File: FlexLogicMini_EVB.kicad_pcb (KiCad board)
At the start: 8 copper layers, 50 x 50 mm, 183 parts, among them IC1 SL2.1s, IC2 MT9700, IC3 MTS4P, IC4 LCMXO2-1200HC-4SG32I, IC5 W25Q16JVUXIQ, J1 GT-USB-7010ASV, J10 Conn_02x03_Odd_Even, J11 Conn_01x04, J12 1.0-3PWB, J13 1.0-3PWB, J2 WJ126V-5.0-2P, J3 WJ126V-5.0-2P, J4 WJ126V-5.0-2P, J5 WJ126V-5.0-2P, J6 Conn_02x03_Odd_Even, J7 Conn_02x03_Odd_Even, J8 Conn_02x03_Odd_Even, J9 Conn_02x03_Odd_Even, SW1 DSWB02LHGETB, U1 ADS1115IDGSR, U10 RP2040, U11 TMUX1574DYYR, U2 ADS1115IDGSR, U3 RQ12000160, U4 RT5752BHGJ5, U5 93LC56BT-I, U6 RQ12000160, U7 FT2232HL, U8 RQ12000160, U9 TLV803SDBZR

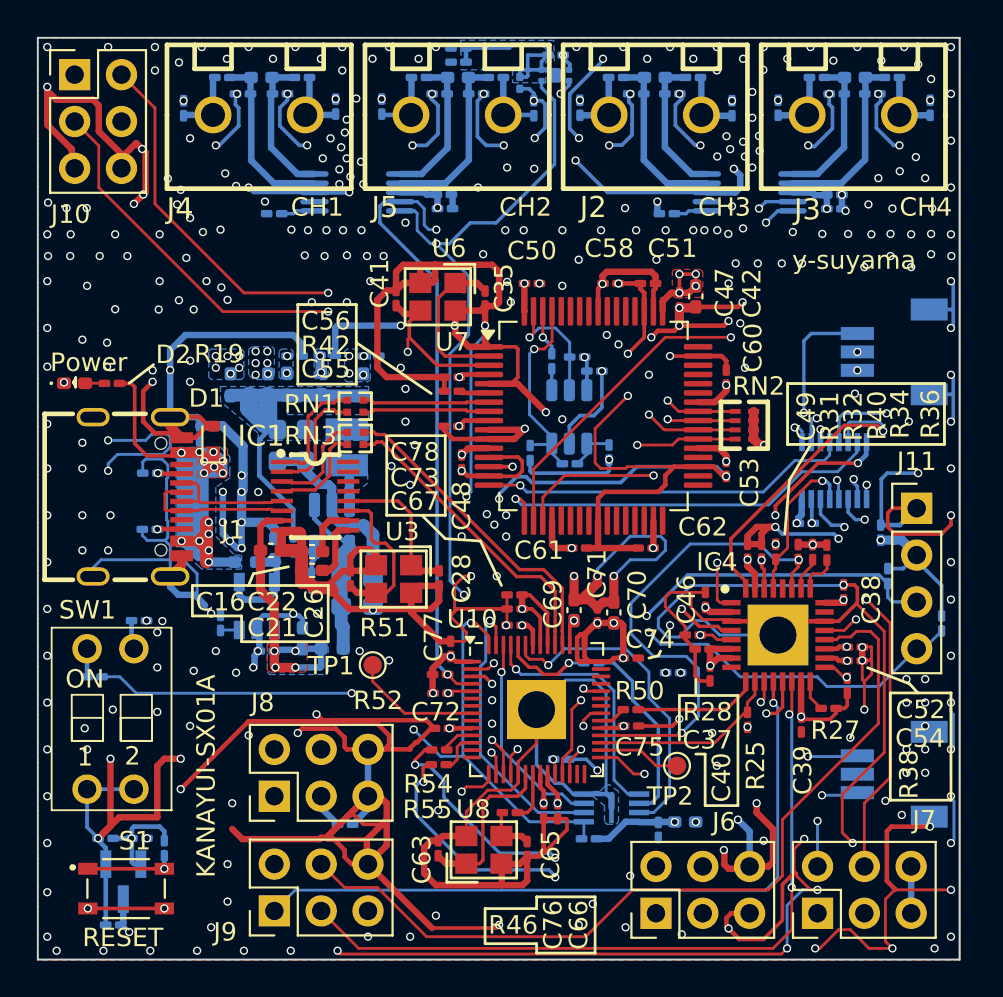
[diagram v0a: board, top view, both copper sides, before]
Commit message: V3 commit
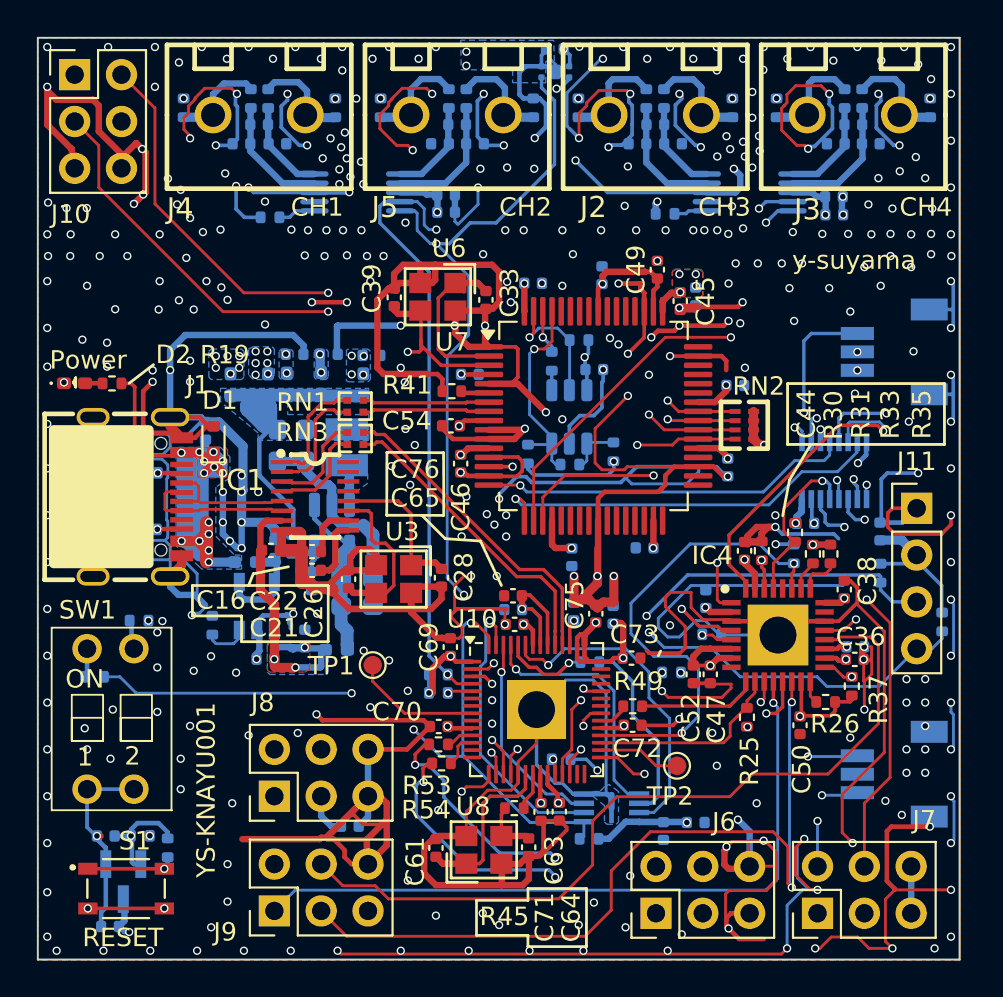
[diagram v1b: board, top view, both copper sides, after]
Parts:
- removed the C31 at (134.3, 72.3)
- removed the C34 at (141.7, 89.1)
- removed the C40 at (148.0, 105.5)
- removed the C66 at (139.7, 113.0)
- removed C78, C79: 0.1uF, Capacitor_SMD:C_0201_0603Metric_Pad0.64x0.40mm_HandSolder
- removed the R27 at (154.4, 107.4)
- removed the R36 at (154.3, 98.9)
- removed the R40 at (152.7, 98.9)
- removed the R52 at (133.3, 106.6)
- removed the R55 at (133.3, 110.4)
- added C33: 33pF, Capacitor_SMD:C_0402_1005Metric, F.Cu at (135.8, 85.2)
- added C36: 0.1uF, Capacitor_SMD:C_0402_1005Metric, F.Cu at (155.8, 104.7)
- added C42: 0.1uF, Capacitor_SMD:C_0402_1005Metric, B.Cu at (127.3, 88.2)
- added C68: 1uF, Capacitor_SMD:C_0402_1005Metric, B.Cu at (142.7, 102.3)
- added R30: 2.2k, Resistor_SMD:R_0402_1005Metric, F.Cu at (150.8, 98.8)
- added R37: 10k, Resistor_SMD:R_0402_1005Metric, F.Cu at (155.7, 106.2)
- added R44: 100, Resistor_SMD:R_0402_1005Metric, B.Cu at (145.9, 105.4)
- added R53: 100, Resistor_SMD:R_0402_1005Metric, F.Cu at (133.2, 109.3)
- C1, C10, C11, C12, C13, C14, C17, C18, C19, C20, C23, C25, C30, C38, C43, C46, C47, C49, C50, C52, C54, C59, C6, C7, C71, C72, C73, C75, C76, C8, C9: footprint Capacitor_SMD:C_0201_0603Metric_Pad0.64x0.40mm_HandSolder -> Capacitor_SMD:C_0402_1005Metric
- C15, C16, C2, C21, C22, C24, C3, C4, C5: footprint Capacitor_SMD:C_0402_1005Metric_Pad0.74x0.62mm_HandSolder -> Capacitor_SMD:C_0402_1005Metric
- C26, C28, C63: value 30pF -> 33pF; footprint Capacitor_SMD:C_0201_0603Metric_Pad0.64x0.40mm_HandSolder -> Capacitor_SMD:C_0402_1005Metric
- C32: value 1000pF -> 0.1uF; footprint Capacitor_SMD:C_0201_0603Metric -> Capacitor_SMD:C_0402_1005Metric
- C35, C41: value 30pF -> 0.1uF; footprint Capacitor_SMD:C_0201_0603Metric_Pad0.64x0.40mm_HandSolder -> Capacitor_SMD:C_0402_1005Metric; moved to B.Cu
- C37, C48, C51, C53, C56, C58, C60, C62, C74, C77: footprint Capacitor_SMD:C_0201_0603Metric_Pad0.64x0.40mm_HandSolder -> Capacitor_SMD:C_0402_1005Metric; moved to B.Cu
- C39, C61: value 0.1uF -> 33pF; footprint Capacitor_SMD:C_0201_0603Metric_Pad0.64x0.40mm_HandSolder -> Capacitor_SMD:C_0402_1005Metric
- C40: renamed from C42; footprint Capacitor_SMD:C_0402_1005Metric_Pad0.74x0.62mm_HandSolder -> Capacitor_SMD:C_0402_1005Metric; moved to B.Cu
- C44, C45, C64: footprint Capacitor_SMD:C_0201_0603Metric_Pad0.64x0.40mm_HandSolder -> Capacitor_SMD:C_0402_1005Metric; moved to F.Cu
- C55, C67: value 0.1uF -> 1uF; footprint Capacitor_SMD:C_0201_0603Metric_Pad0.64x0.40mm_HandSolder -> Capacitor_SMD:C_0402_1005Metric; moved to B.Cu
- C57, C69, C70: value 1uF -> 0.1uF; footprint Capacitor_SMD:C_0402_1005Metric_Pad0.74x0.62mm_HandSolder -> Capacitor_SMD:C_0402_1005Metric
- C65: value 30pF -> 0.1uF; footprint Capacitor_SMD:C_0201_0603Metric_Pad0.64x0.40mm_HandSolder -> Capacitor_SMD:C_0402_1005Metric
- C66: renamed from C68; footprint Capacitor_SMD:C_0201_0603Metric_Pad0.64x0.40mm_HandSolder -> Capacitor_SMD:C_0402_1005Metric
- R1, R17, R18, R19, R2, R20, R21, R22, R23, R24, R25, R3, R31, R39, R4, R5, R54, R6, R7, R8: footprint Resistor_SMD:R_0201_0603Metric_Pad0.64x0.40mm_HandSolder -> Resistor_SMD:R_0402_1005Metric
- R10, R11, R12, R13, R14, R15, R16, R9: value 240 -> 220; footprint Resistor_SMD:R_0201_0603Metric_Pad0.64x0.40mm_HandSolder -> Resistor_SMD:R_0402_1005Metric
- R26: value 0 -> 10k; footprint Resistor_SMD:R_0201_0603Metric_Pad0.64x0.40mm_HandSolder -> Resistor_SMD:R_0402_1005Metric; moved to F.Cu
- R27: renamed from R28; footprint Resistor_SMD:R_0201_0603Metric_Pad0.64x0.40mm_HandSolder -> Resistor_SMD:R_0402_1005Metric; moved to B.Cu
- R28: renamed from R29; footprint Resistor_SMD:R_0201_0603Metric_Pad0.64x0.40mm_HandSolder -> Resistor_SMD:R_0402_1005Metric
- R29: renamed from R30; footprint Resistor_SMD:R_0201_0603Metric_Pad0.64x0.40mm_HandSolder -> Resistor_SMD:R_0402_1005Metric
- R32: value 2.2k -> 10k; footprint Resistor_SMD:R_0201_0603Metric_Pad0.64x0.40mm_HandSolder -> Resistor_SMD:R_0402_1005Metric; moved to B.Cu
- R33, R35: value 10k -> 4.7k; footprint Resistor_SMD:R_0201_0603Metric_Pad0.64x0.40mm_HandSolder -> Resistor_SMD:R_0402_1005Metric; moved to F.Cu
- R34: value 4.7k -> 10k; footprint Resistor_SMD:R_0201_0603Metric_Pad0.64x0.40mm_HandSolder -> Resistor_SMD:R_0402_1005Metric; moved to B.Cu
- R36: renamed from R37; footprint Resistor_SMD:R_0201_0603Metric_Pad0.64x0.40mm_HandSolder -> Resistor_SMD:R_0402_1005Metric
- R38, R51: footprint Resistor_SMD:R_0201_0603Metric_Pad0.64x0.40mm_HandSolder -> Resistor_SMD:R_0402_1005Metric; moved to B.Cu
- R40: renamed from R41; value 30 -> 33; footprint Resistor_SMD:R_0201_0603Metric_Pad0.64x0.40mm_HandSolder -> Resistor_SMD:R_0402_1005Metric
- R41: renamed from R42; footprint Resistor_SMD:R_0201_0603Metric_Pad0.64x0.40mm_HandSolder -> Resistor_SMD:R_0402_1005Metric
- R42: renamed from R43; footprint Resistor_SMD:R_0201_0603Metric_Pad0.64x0.40mm_HandSolder -> Resistor_SMD:R_0402_1005Metric
- R43: renamed from R44; footprint Resistor_SMD:R_0201_0603Metric_Pad0.64x0.40mm_HandSolder -> Resistor_SMD:R_0402_1005Metric
- R45: value 100 -> 33; footprint Resistor_SMD:R_0201_0603Metric_Pad0.64x0.40mm_HandSolder -> Resistor_SMD:R_0402_1005Metric; moved to F.Cu
- R46: value 30 -> 33; footprint Resistor_SMD:R_0201_0603Metric_Pad0.64x0.40mm_HandSolder -> Resistor_SMD:R_0402_1005Metric; moved to B.Cu
- R47: value 30 -> 10k; footprint Resistor_SMD:R_0201_0603Metric_Pad0.64x0.40mm_HandSolder -> Resistor_SMD:R_0402_1005Metric
- R48: value 10k -> 33; footprint Resistor_SMD:R_0201_0603Metric_Pad0.64x0.40mm_HandSolder -> Resistor_SMD:R_0402_1005Metric
- R49: value 30 -> 33; footprint Resistor_SMD:R_0201_0603Metric_Pad0.64x0.40mm_HandSolder -> Resistor_SMD:R_0402_1005Metric; moved to F.Cu
- R50: value 30 -> 2.2k; footprint Resistor_SMD:R_0201_0603Metric_Pad0.64x0.40mm_HandSolder -> Resistor_SMD:R_0402_1005Metric; moved to B.Cu
- R52: renamed from R53; footprint Resistor_SMD:R_0201_0603Metric_Pad0.64x0.40mm_HandSolder -> Resistor_SMD:R_0402_1005Metric
- R55: renamed from R56; footprint Resistor_SMD:R_0201_0603Metric_Pad0.64x0.40mm_HandSolder -> Resistor_SMD:R_0402_1005Metric
- moved R26 40.7 mm to (154.2, 107.0), turned to 180 degrees
- moved C62 35.6 mm to (115.4, 119.2)
- moved C39 32.0 mm to (130.8, 85.1), turned to 90 degrees
- moved C50 28.0 mm to (152.8, 108.3), turned to -90 degrees
- moved R49 26.5 mm to (143.8, 107.3), turned to 0 degrees
- moved R47 26.2 mm to (117.1, 114.3)
- moved C54 25.3 mm to (133.9, 92.0), turned to 180 degrees
- moved C55 25.3 mm to (147.2, 113.6)
- moved C44 25.0 mm to (149.8, 98.8), turned to 90 degrees
- moved C64 25.0 mm to (139.8, 113.0), turned to -90 degrees
- moved C59 24.5 mm to (149.3, 89.9), turned to 0 degrees
- moved R38 23.7 mm to (140.9, 87.4), turned to 180 degrees
- moved C77 20.4 mm to (153.1, 97.3), turned to 0 degrees
- moved C47 20.4 mm to (148.0, 105.5)
- moved C35 20.2 mm to (147.7, 101.4)
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- renumbered C33 to C31, C36 to C34
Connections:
- C30 pad 2: TMPGND -> GND
- C32 pad 1: GND -> +3.3V_FT2232H
- C32 pad 2: TMPGND -> GND
- C35 pad 1: GND -> +3.3V_D
- C35 pad 2: Net-(U6-OSC) -> GND
- C39 pad 1: +3.3V_D -> CLK12M
- C41 pad 1: CLK12M -> +3.3V_A_FT2232H
- C43 pad 1: +3.3V_A_FT2232H -> +3.3V_EXT
- C44 pad 1: +3.3V_ADC -> +3.3V_D
- C45 pad 1: +3.3V_EXT -> VCORE_FT2232H
- C46 pad 1: +3.3V_D -> VCORE_FT2232H
- C47 pad 1: VCORE_FT2232H -> +3.3V_D
- C49 pad 1: +3.3V_D -> +3.3V_FT2232H
- C50 pad 1: VCORE_FT2232H -> +3.3V_D
- C51 pad 1: +3.3V_FT2232H -> VCORE_FT2232H
- C53 pad 1: VCORE_FT2232H -> +3.3V_A_FT2232H
- C54 pad 1: +3.3V_D -> +3.3V_A_FT2232H
- C55 pad 1: +3.3V_A_FT2232H -> GND
- C55 pad 2: GND -> +3.3V_D
- C56 pad 1: +3.3V_A_FT2232H -> +3.3V_FT2232H
- C57 pad 1: GND -> +3.3V_D
- C57 pad 2: +3.3V_D -> GND
- C59 pad 1: +3.3V_D -> +3.3V_FT2232H
- C61 pad 1: +3.3V_FT2232H -> GND
- C61 pad 2: GND -> Net-(U10-XIN)
- C62 pad 1: +3.3V_FT2232H -> VBUS
- C63 pad 1: GND -> Net-(U8-OSC2)
- C63 pad 2: Net-(U10-XIN) -> GND
- C64 pad 1: VBUS -> +1.1V_MCU
- C65 pad 1: Net-(U8-OSC2) -> +1.1V_MCU
- C67 pad 1: +1.1V_MCU -> GND
- C67 pad 2: GND -> +1.1V_MCU
- C69 pad 1: GND -> +3.3V_D
- C69 pad 2: +1.1V_MCU -> GND
- C70 pad 1: GND -> +3.3V_D
- C70 pad 2: +3.3V_D -> GND
- IC3 pad 2: TMPGND -> GND
- IC3 pad 5: TMPGND -> GND
- R26 pad 1: GND -> +3.3V_D
- R26 pad 2: TMPGND -> Net-(IC4-PB20C)
- R31 pad 1: TCK_FPGA -> +3.3V_D
- R31 pad 2: GND -> TMS_FPGA
- R32 pad 1: +3.3V_D -> +3.3V_FT2232H
- R32 pad 2: TMS_FPGA -> Net-(U5-DO)
- R33 pad 1: +3.3V_FT2232H -> +3.3V_D
- R33 pad 2: Net-(U5-DO) -> Net-(IC4-PT15C)
- R34 pad 1: +3.3V_D -> +3.3V_FT2232H
- R34 pad 2: Net-(IC4-PT15C) -> Net-(U5-DI)
- R35 pad 1: +3.3V_FT2232H -> +3.3V_D
- R35 pad 2: Net-(U5-DI) -> Net-(IC4-PT15D)
- R38 pad 1: +3.3V_D -> +3.3V_FT2232H
- R38 pad 2: SPI0_MOSI -> Net-(U5-CS)
- R39 pad 1: +3.3V_FT2232H -> +3.3V_D
- R39 pad 2: Net-(U5-CS) -> SPI0_CS_N
- R45 pad 1: Net-(J12-Pad3) -> Net-(U8-OSC2)
- R45 pad 2: Net-(U10-SWD) -> Net-(U10-XOUT)
- R46 pad 1: Net-(U8-OSC2) -> QSPI_SCLK
- R46 pad 2: Net-(U10-XOUT) -> Net-(U10-QSPI_SCLK)
- R47 pad 1: QSPI_SCLK -> +3.3V_D
- R47 pad 2: Net-(U10-QSPI_SCLK) -> RESET_N
- R48 pad 1: +3.3V_D -> RESET_N
- R48 pad 2: RESET_N -> Net-(R48-Pad2)
- R49 pad 1: RESET_N -> Net-(U10-GPIO22)
- R49 pad 2: Net-(R49-Pad2) -> SPI0_CLK
- R50 pad 1: Net-(U10-GPIO22) -> +3.3V_D
- R50 pad 2: SPI0_CLK -> I2CSDA_ADC
- R51 pad 2: I2CSDA_ADC -> I2CSCL_ADC
- R54 pad 1: Net-(J13-Pad1) -> Net-(U10-GPIO9)
- R54 pad 2: Net-(U10-GPIO8) -> Net-(J13-Pad3)
- S1 pad 1: Net-(R49-Pad2) -> Net-(R48-Pad2)
- S1 pad 2: Net-(R49-Pad2) -> Net-(R48-Pad2)
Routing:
- net GND: track 1299.1 -> 1227.2 mm, vias 376 -> 388
- net +3.3V_D: track 173.3 -> 202.6 mm, vias 29 -> 28
- net +1.1V_MCU: track 4.74 -> 25.7 mm
- net VCORE_FT2232H: track 59.1 -> 41.4 mm
- net +3.3V_FT2232H: track 92.8 -> 107.4 mm
- net EVBDET_N: track 34.7 -> 21.5 mm
- net +3.3V_A_FT2232H: track 4.36 -> 17.3 mm
- net TMPGND: track 11.9 -> 0.00 mm
- net RESET_N: track 85.0 -> 77.1 mm
- net Net-(R49-Pad2): track 4.86 -> 0.00 mm, vias 1 -> 0
- net Net-(R48-Pad2): track 0.00 -> 4.86 mm, vias 0 -> 1
- net VBUS: track 37.7 -> 42.5 mm, vias 5 -> 4
- net FPGA_IO3: track 40.5 -> 43.4 mm
- net Net-(U2-AIN3): track 9.97 -> 7.11 mm
- net Net-(U2-AIN0): track 9.56 -> 6.71 mm
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- added copper zone on B.Cu, net VCORE_FT2232H
- removed copper zone on In5.Cu, net +1.1V_MCU
- removed copper zone on In5.Cu, net +3.3V_A_FT2232H
- removed copper zone on B.Cu, net TMPGND
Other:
- board text added: "YS-KNAYU001"
- board text removed: "GND +3.3V SCL SDA"
- board text removed: "KANAYUI-SX01A"
